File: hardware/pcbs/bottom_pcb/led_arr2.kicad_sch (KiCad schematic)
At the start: 21 parts

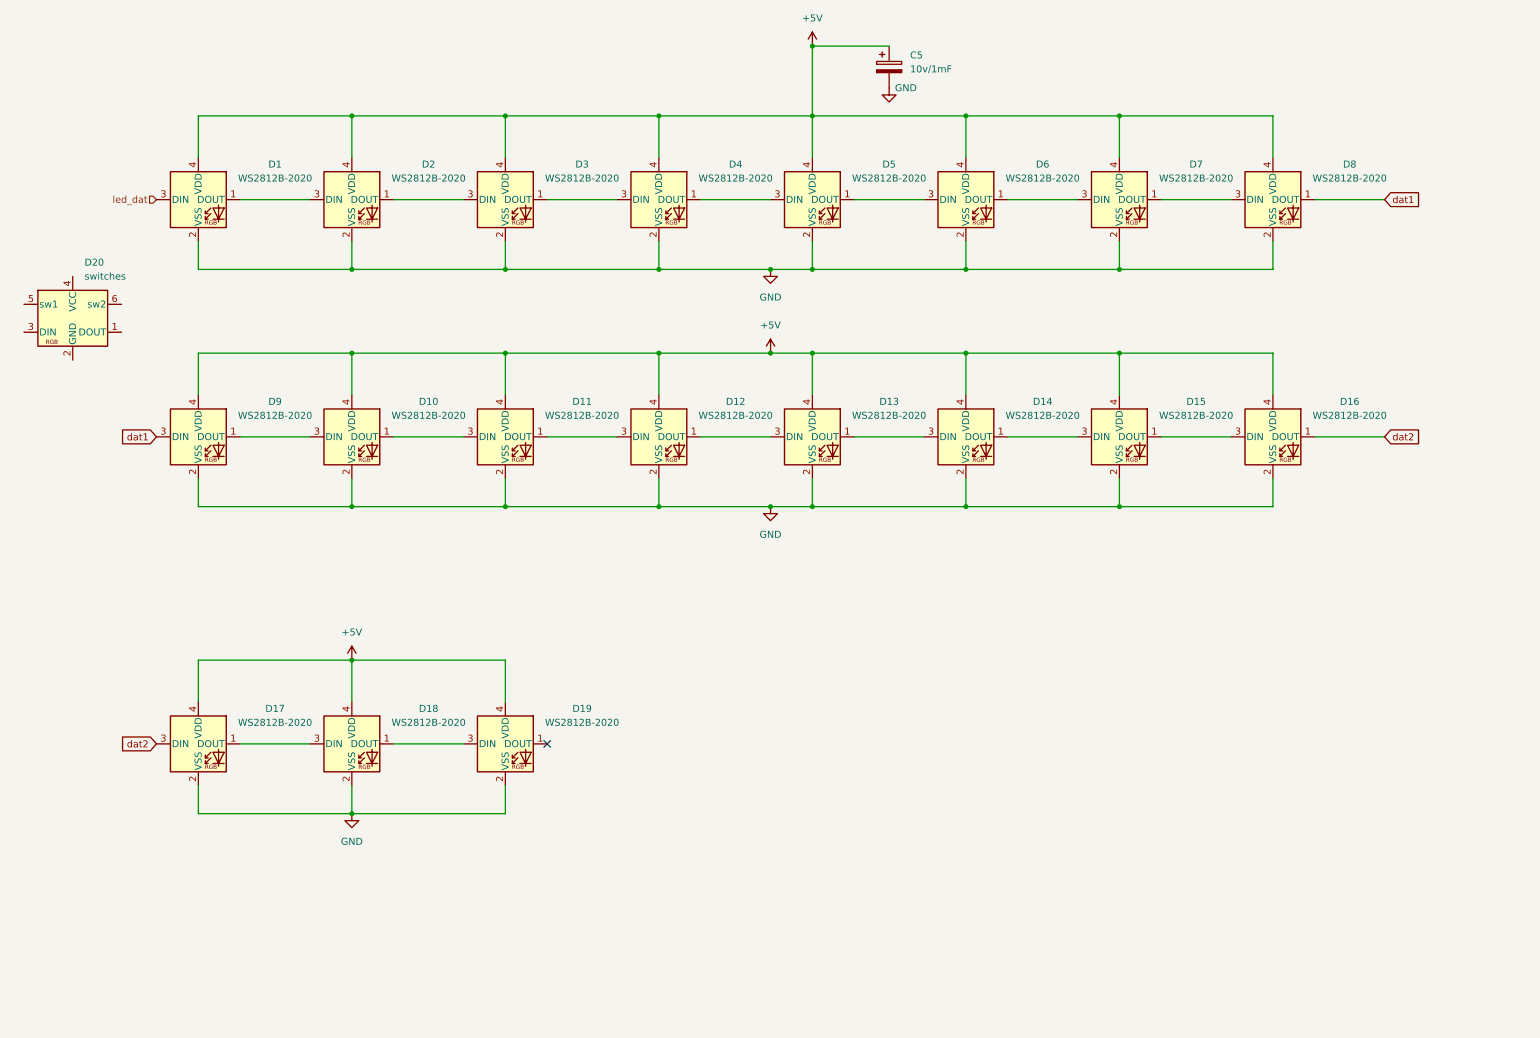
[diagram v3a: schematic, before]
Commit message: t
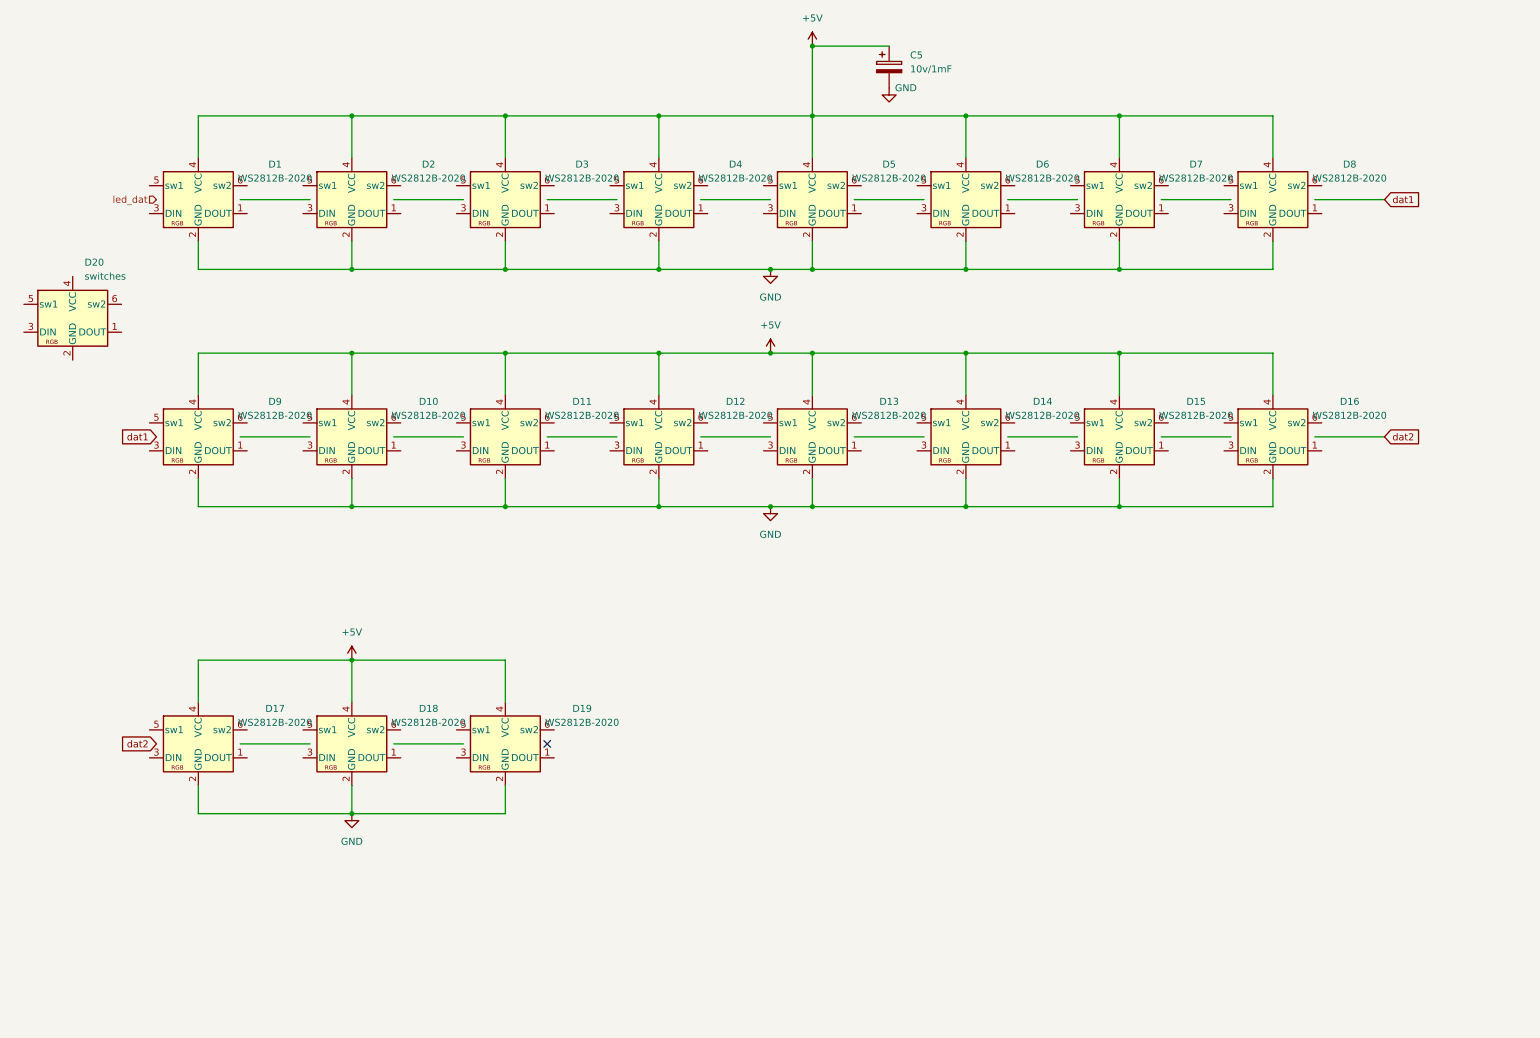
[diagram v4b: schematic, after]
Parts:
- D1, D10, D11, D12, D13, D14, D15, D16, D17, D18, D19, D2, D3, D4, D5, D6, D7, D8, D9: symbol LED:WS2812B-2020 -> 3dAudioSym:A3_switches_led
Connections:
- net dat1: no longer D8.1 (DOUT), D9.3 (DIN)
- net dat2: no longer D16.1 (DOUT), D17.3 (DIN)
- net led_dat: no longer D1.3 (DIN)
- net at D13.1 (DOUT): no longer D14.3 (DIN)
- net at D13.3 (DIN): no longer D12.1 (DOUT)
- net at D15.1 (DOUT): no longer D16.3 (DIN)
- net at D15.3 (DIN): no longer D14.1 (DOUT)
- net at D1.1 (DOUT): no longer D2.3 (DIN)
- net at D18.1 (DOUT): no longer D19.3 (DIN)
- net at D18.3 (DIN): no longer D17.1 (DOUT)
- net at D8.3 (DIN): no longer D7.1 (DOUT)
- net at D10.1 (DOUT): no longer D11.3 (DIN)
- net at D10.3 (DIN): no longer D9.1 (DOUT)
- net at D4.1 (DOUT): no longer D5.3 (DIN)
- net at D4.3 (DIN): no longer D3.1 (DOUT)
- net at D11.1 (DOUT): no longer D12.3 (DIN)
- net at D2.1 (DOUT): no longer D3.3 (DIN)
- net at D5.1 (DOUT): no longer D6.3 (DIN)
- net at D7.3 (DIN): no longer D6.1 (DOUT)
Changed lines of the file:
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@@
 	)
 	(symbol
-		(lib_id "LED:WS2812B-2020")
+		(lib_id "3dAudioSym:A3_switches_led")
 		(at 160.02 88.9 0)
 		(unit 1)
@@
 	)
 	(symbol
-		(lib_id "LED:WS2812B-2020")
+		(lib_id "3dAudioSym:A3_switches_led")
 		(at 215.9 88.9 0)
 		(unit 1)
@@
 	)
 	(symbol
-		(lib_id "LED:WS2812B-2020")
+		(lib_id "3dAudioSym:A3_switches_led")
 		(at 48.26 45.72 0)
 		(unit 1)
@@
 	)
 	(symbol
-		(lib_id "LED:WS2812B-2020")
+		(lib_id "3dAudioSym:A3_switches_led")
 		(at 76.2 144.78 0)
 		(unit 1)
@@
 	)
 	(symbol
-		(lib_id "LED:WS2812B-2020")
+		(lib_id "3dAudioSym:A3_switches_led")
 		(at 243.84 45.72 0)
 		(unit 1)
@@
 	)
 	(symbol
-		(lib_id "LED:WS2812B-2020")
+		(lib_id "3dAudioSym:A3_switches_led")
 		(at 76.2 88.9 0)
 		(unit 1)
@@
 	)
 	(symbol
-		(lib_id "LED:WS2812B-2020")
+		(lib_id "3dAudioSym:A3_switches_led")
 		(at 132.08 45.72 0)
 		(unit 1)
@@
 	)
 	(symbol
-		(lib_id "LED:WS2812B-2020")
+		(lib_id "3dAudioSym:A3_switches_led")
 		(at 104.14 144.78 0)
 		(unit 1)
@@
 	)
 	(symbol
-		(lib_id "LED:WS2812B-2020")
+		(lib_id "3dAudioSym:A3_switches_led")
 		(at 104.14 88.9 0)
 		(unit 1)
@@
 	)
 	(symbol
-		(lib_id "LED:WS2812B-2020")
+		(lib_id "3dAudioSym:A3_switches_led")
 		(at 76.2 45.72 0)
 		(unit 1)
@@
 	)
 	(symbol
-		(lib_id "LED:WS2812B-2020")
+		(lib_id "3dAudioSym:A3_switches_led")
 		(at 187.96 88.9 0)
 		(unit 1)
@@
 	)
 	(symbol
-		(lib_id "LED:WS2812B-2020")
+		(lib_id "3dAudioSym:A3_switches_led")
 		(at 160.02 45.72 0)
 		(unit 1)
@@
 	)
 	(symbol
-		(lib_id "LED:WS2812B-2020")
+		(lib_id "3dAudioSym:A3_switches_led")
 		(at 215.9 45.72 0)
 		(unit 1)
@@
 	)
 	(symbol
-		(lib_id "LED:WS2812B-2020")
+		(lib_id "3dAudioSym:A3_switches_led")
 		(at 243.84 88.9 0)
 		(unit 1)
@@
 	)
 	(symbol
-		(lib_id "LED:WS2812B-2020")
+		(lib_id "3dAudioSym:A3_switches_led")
 		(at 48.26 88.9 0)
 		(unit 1)
@@
 	)
 	(symbol
-		(lib_id "LED:WS2812B-2020")
+		(lib_id "3dAudioSym:A3_switches_led")
 		(at 104.14 45.72 0)
 		(unit 1)
@@
 	)
 	(symbol
-		(lib_id "LED:WS2812B-2020")
+		(lib_id "3dAudioSym:A3_switches_led")
 		(at 187.96 45.72 0)
 		(unit 1)
@@
 	)
 	(symbol
-		(lib_id "LED:WS2812B-2020")
+		(lib_id "3dAudioSym:A3_switches_led")
 		(at 48.26 144.78 0)
 		(unit 1)
@@
 	)
 	(symbol
-		(lib_id "LED:WS2812B-2020")
+		(lib_id "3dAudioSym:A3_switches_led")
 		(at 132.08 88.9 0)
 		(unit 1)
